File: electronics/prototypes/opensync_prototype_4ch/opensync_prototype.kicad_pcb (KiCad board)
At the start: 4 copper layers, 100 x 100 mm, 86 parts, among them J1 61400416121, J12 SM03B-SRSS-TB, J13 61611042121502, J2 61611042121502, J4 61611042121502, J5 61611042121502, J6 61611042121502, J7 61611042121502, SW1 SW_Push, SW2 SW_Push, U1 NCP1117-3.3_SOT223, U2 RP2354_80QFN, U3 NXE2S0505MC, U4 SN74LVC1G17DCKR, U5 SN74LVC1T45DCKR, U6 SN74LVC1T45DCKR, U7 SN74LVC1T45DCKR, U8 SN74LVC1T45DCKR, Y1 ABM8-272-T3

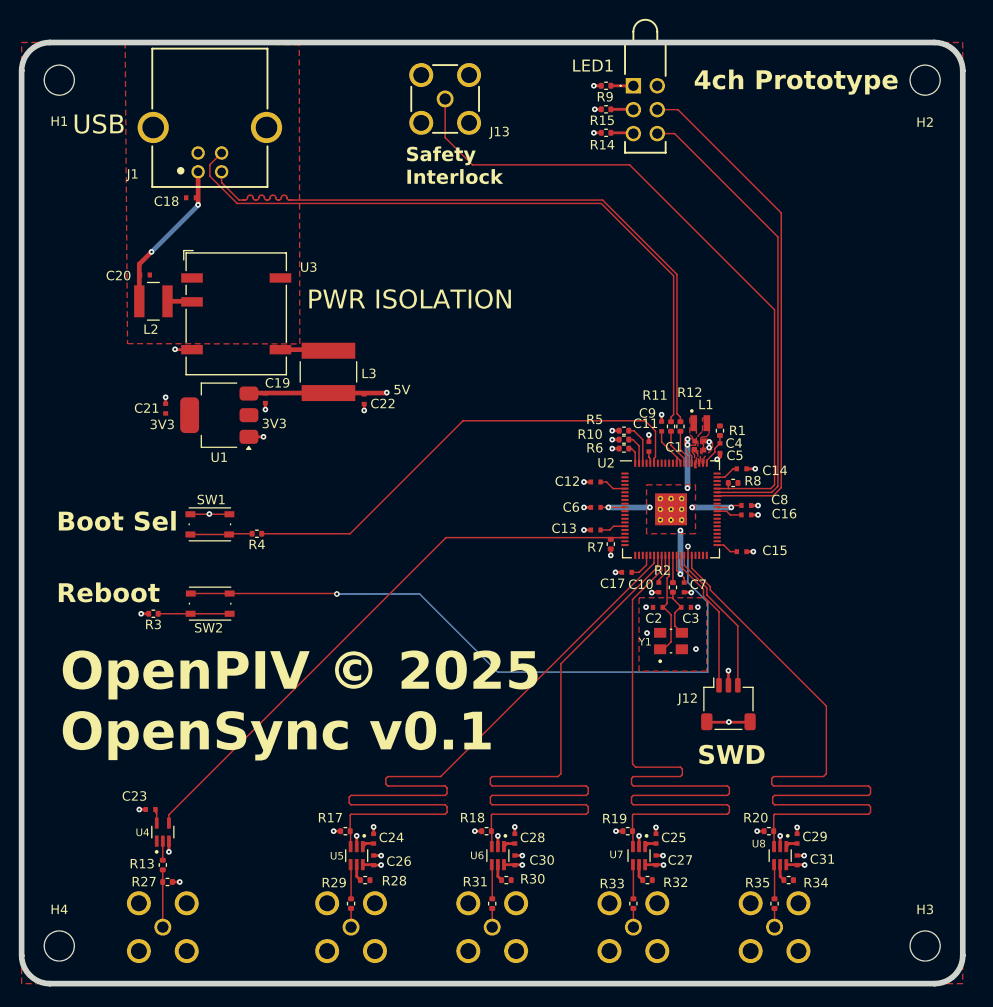
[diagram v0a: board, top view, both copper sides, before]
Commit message: Backup before storm
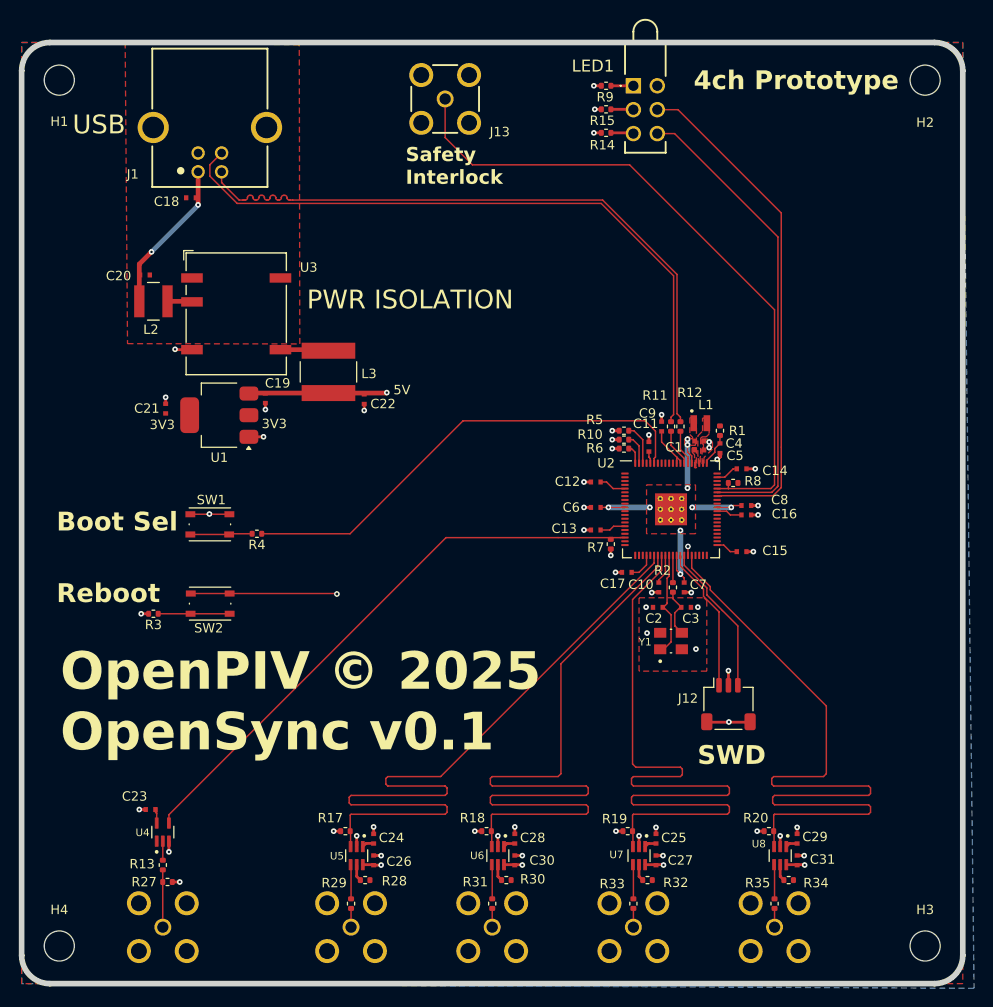
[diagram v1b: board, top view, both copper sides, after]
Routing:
- net /Microcontroller and Ext. Clock/RUN: track 73.6 -> 56.3 mm
- added copper zone on B.Cu, net GND
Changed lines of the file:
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@@
 		(net 44)
 	)
-	(via
+	(via micro
 		(at 95.5 103.6)
 		(size 0.6)
 		(drill 0.3)
-		(layers "F.Cu" "B.Cu")
+		(layers "F.Cu" "In2.Cu")
 		(free yes)
 		(net 44)
 	)
-	(via
+	(via micro
 		(at 132.8 98.55)
 		(size 0.6)
 		(drill 0.3)
-		(layers "F.Cu" "B.Cu")
+		(layers "F.Cu" "In2.Cu")
 		(free yes)
 		(net 44)
 	)
 	(segment
-		(start 134.9 104.5)
-		(end 134.9 111.9)
-		(width 0.1565)
-		(layer "B.Cu")
+		(start 125.3 100.4)
+		(end 98.7 100.4)
+		(width 0.1565)
+		(layer "In2.Cu")
 		(net 44)
 	)
 	(segment
-		(start 134.9 111.9)
-		(end 112.6 111.9)
-		(width 0.1565)
-		(layer "B.Cu")
+		(start 132.119184 100)
+		(end 125.7 100)
+		(width 0.1565)
+		(layer "In2.Cu")
 		(net 44)
 	)
 	(segment
-		(start 132.8 102.4)
-		(end 134.9 104.5)
-		(width 0.1565)
-		(layer "B.Cu")
+		(start 132.8 98.55)
+		(end 132.8 99.319184)
+		(width 0.1565)
+		(layer "In2.Cu")
 		(net 44)
 	)
 	(segment
-		(start 132.8 98.55)
-		(end 132.8 102.4)
-		(width 0.1565)
-		(layer "B.Cu")
+		(start 98.7 100.4)
+		(end 95.5 103.6)
+		(width 0.1565)
+		(layer "In2.Cu")
 		(net 44)
 	)
 	(segment
-		(start 112.6 111.9)
-		(end 104.3 103.6)
-		(width 0.1565)
-		(layer "B.Cu")
+		(start 132.8 99.319184)
+		(end 132.119184 100)
+		(width 0.1565)
+		(layer "In2.Cu")
 		(net 44)
 	)
 	(segment
-		(start 104.3 103.6)
-		(end 95.5 103.6)
-		(width 0.1565)
-		(layer "B.Cu")
+		(start 125.7 100)
+		(end 125.3 100.4)
+		(width 0.1565)
+		(layer "In2.Cu")
 		(net 44)
 	)
@@
 			)
 		)
+	)
+	(zone
+		(net 2)
+		(net_name "GND")
+		(layer "B.Cu")
+		(hatch edge 0.5)
+		(connect_pads
+			(clearance 0.3)
+		)
+		(min_thickness 0.25)
+		(filled_areas_thickness no)
+		(fill yes
+			(thermal_gap 0.5)
+			(thermal_bridge_width 0.5)
+		)
+		(polygon
+			(pts
+				(xy 62 45) (xy 162 45) (xy 163.2 145.5) (xy 62 145)
+			)
+		)
